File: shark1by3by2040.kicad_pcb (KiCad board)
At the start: 2 copper layers, 35 parts, among them J1 SWD, SW1 SW_USB_BOOT, SW2 SW_Reset, U1 RP2040, U2 W25Q128JVS, U3 NCP1117-3.3_SOT223, Y1 ABLS-12.000MHZ-B4-T

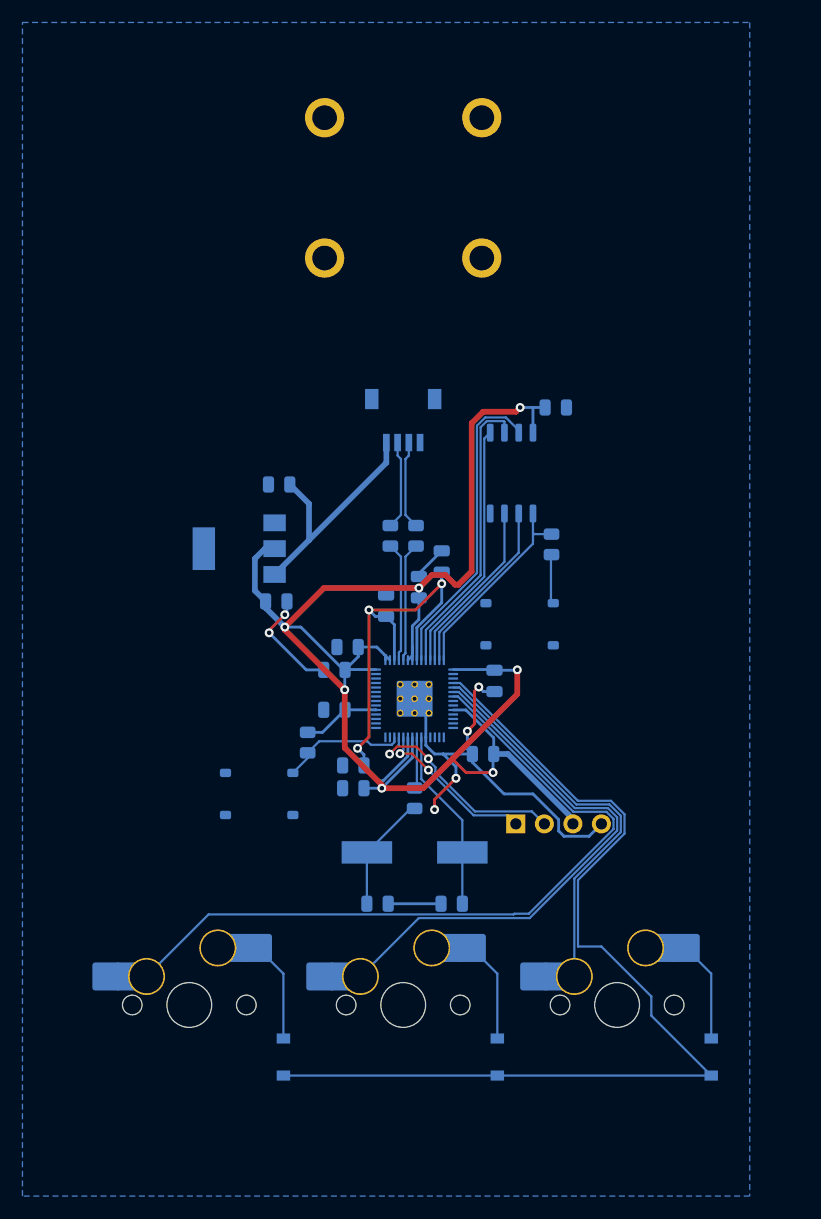
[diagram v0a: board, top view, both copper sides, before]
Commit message: 1by3by2040 rev1
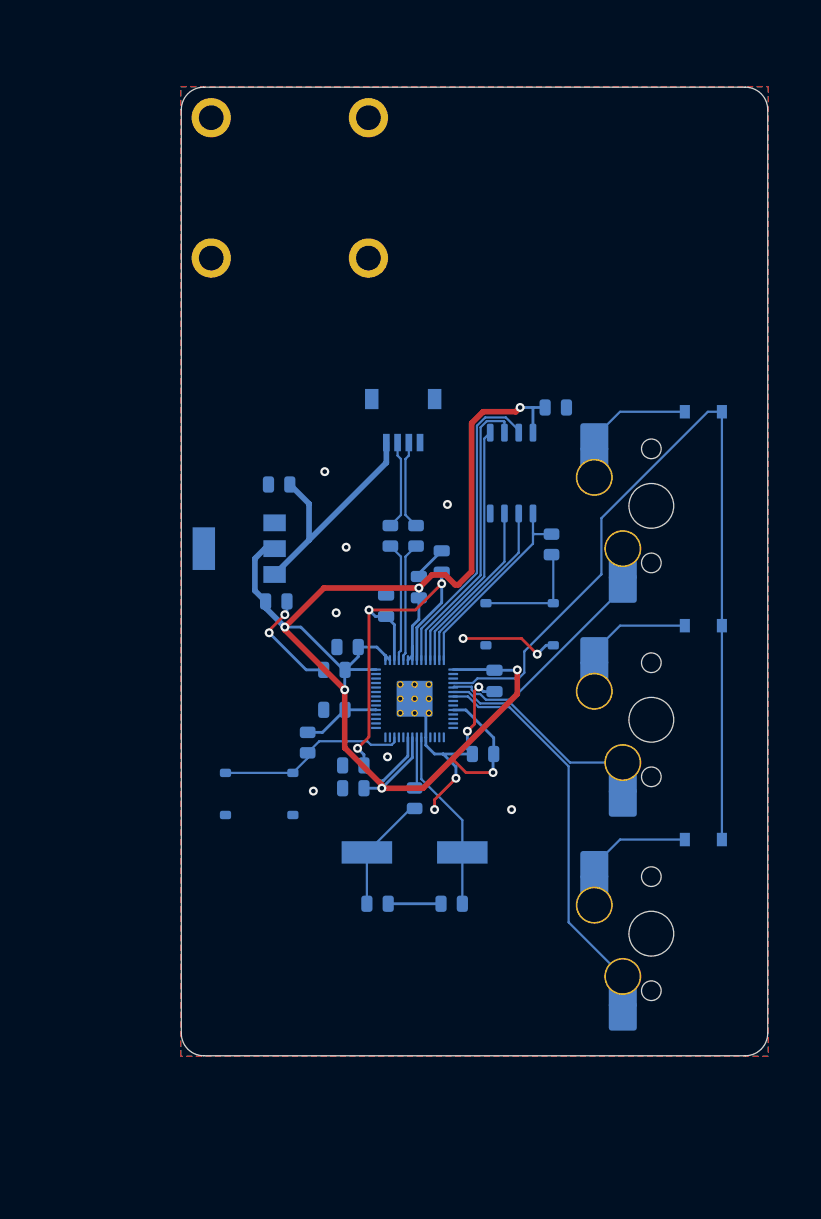
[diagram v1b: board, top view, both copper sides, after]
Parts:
- removed J1: SWD, Connector_PinHeader_2.54mm:PinHeader_1x04_P2.54mm_Vertical
- SW1: value SW_USB_BOOT -> BOOTSEL
- SW2: value SW_Reset -> Reset
- U2: value W25Q128JVS -> W25Q16JVSSIQ
- moved D3 57.5 mm to (200.3, 57.8), turned to 180 degrees
- moved MX3 44.6 mm to (195.7, 66.2), turned to -90 degrees
- moved D2 42.6 mm to (200.3, 76.8), turned to 180 degrees
- moved D1 42.1 mm to (200.3, 95.9), turned to 180 degrees
- moved MX1 41.6 mm to (195.7, 104.3), turned to -90 degrees
- moved MX2 33.7 mm to (195.7, 85.2), turned to -90 degrees
- moved H1 10.1 mm to (163.5, 37.8)
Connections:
- U1 pad 24: Net-(J1-Pad1) -> unconnected-(U1-Pad24)
- U1 pad 25: Net-(J1-Pad2) -> unconnected-(U1-Pad25)
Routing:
- net col0: track 66.7 -> 33.6 mm
- net col1: track 48.7 -> 17.7 mm
- net Net-(J1-Pad2): track 19.1 -> 0.00 mm, vias 2 -> 0
- net col2: track 35.7 -> 19.9 mm
- net Net-(J1-Pad1): track 14.5 -> 0.00 mm, vias 2 -> 0
- net row0: track 89.3 -> 76.1 mm
- net +3V3: track 155.9 -> 145.9 mm
- net GND: track 55.3 -> 48.0 mm, vias 6 -> 15
- net Net-(R3-Pad1): track 4.07 -> 10.2 mm
- net Net-(R5-Pad2): track 11.1 -> 17.1 mm
- added copper zone on F.Cu, net GND
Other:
- board outline added: 52.2 x 86.3 mm

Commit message: 1by3by2040 rev2
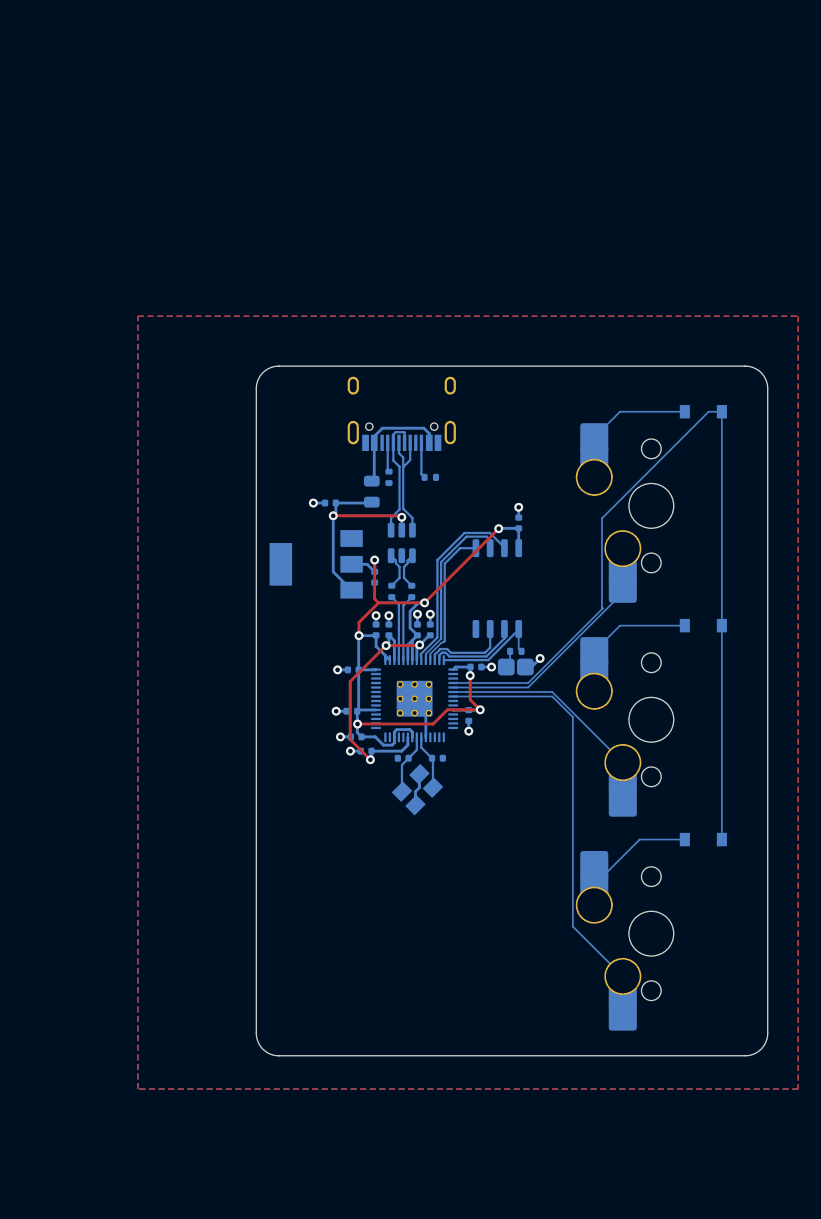
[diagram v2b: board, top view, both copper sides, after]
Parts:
- removed A1: USB, random-keyboard-parts:JST-SR-4
- removed H1: Daughterboard, local:UNIFIED-DAUGHTERBOARD-C3
- removed SW1: BOOTSEL, local:TS-1187A
- removed SW2: Reset, local:TS-1187A
- added F1: 500mA, Fuse:Fuse_0805_2012Metric, B.Cu at (170.8, 64.9)
- added JP1: BOOTSEL, random-keyboard-parts:Jumper-UserFriendly-Small, B.Cu at (183.6, 80.5)
- added U4: USBLC6-2SC6, Package_TO_SOT_SMD:SOT-23-6, B.Cu at (173.5, 69.5)
- added USB1: HRO-TYPE-C-31-M-12, Type-C:HRO-TYPE-C-31-M-12-Assembly, B.Cu at (173.5, 52.9)
- C1, C10, C11, C12, C13, C14, C15, C2, C3, C4, C5, C6, C7: footprint Capacitor_SMD:C_0805_2012Metric -> Capacitor_SMD:C_0402_1005Metric
- C16, C17: value 27pF -> 22pF; footprint Capacitor_SMD:C_0805_2012Metric -> Capacitor_SMD:C_0402_1005Metric
- D1, D2, D3: footprint Diode_SMD:D_SOD-123 -> random-keyboard-parts:D_SOD-123-Pretty
- R1, R2, R3: footprint Resistor_SMD:R_0805_2012Metric -> Resistor_SMD:R_0402_1005Metric
- R4, R5: value 1k -> 5.1k; footprint Resistor_SMD:R_0805_2012Metric -> Resistor_SMD:R_0402_1005Metric
- Y1: value ABLS-12.000MHZ-B4-T -> RH100-12.000-16-3030-TR; footprint Crystal:Crystal_SMD_HC49-SD -> Crystal:Crystal_SMD_3225-4Pin_3.2x2.5mm
- moved R4 28.7 mm to (172.3, 63.6), turned to -90 degrees
- moved R5 26.0 mm to (176.0, 63.6), turned to 0 degrees
- moved C17 13.2 mm to (173.6, 88.6)
- moved C16 13.0 mm to (176.7, 88.6)
- moved C13 10.8 mm to (183.9, 67.7), turned to 90 degrees
- moved U2 10.4 mm to (182.0, 73.5)
- moved R3 10.0 mm to (183.6, 79.1), turned to 0 degrees
- moved C14 9.03 mm to (171.1, 72.5), turned to 90 degrees
- moved U3 7.00 mm to (165.9, 71.4)
- moved C1 6.18 mm to (176.0, 77.2)
- moved Y1 5.59 mm to (174.9, 91.4), turned to 45 degrees
- moved R1 4.97 mm to (174.4, 73.8)
- moved R2 4.95 mm to (172.6, 73.8)
- moved C15 4.86 mm to (167.1, 65.9)
- moved C5 4.58 mm to (169.4, 86.7)
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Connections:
- net /DN renamed Net-(R2-Pad1)
- net /DP renamed Net-(R1-Pad1)
- C16 pad 1: GND -> XIN
- C16 pad 2: Net-(C16-Pad2) -> GND
- C17 pad 1: GND -> XOUT
- C17 pad 2: Net-(C17-Pad2) -> GND
- R4 pad 1: Net-(C17-Pad2) -> Net-(R4-Pad1)
- R4 pad 2: Net-(R4-Pad2) -> GND
- R5 pad 1: +3V3 -> Net-(R5-Pad1)
- R5 pad 2: Net-(R5-Pad2) -> GND
- U1 pad 20: Net-(C16-Pad2) -> XIN
- U1 pad 21: Net-(R4-Pad2) -> XOUT
- U1 pad 26: Net-(R5-Pad2) -> +3V3
- Y1 pad 1: Net-(C17-Pad2) -> XOUT
- Y1 pad 2: Net-(C16-Pad2) -> GND
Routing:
- net +3V3: track 145.9 -> 79.7 mm
- net GND: track 48.0 -> 17.1 mm, vias 15 -> 13
- net +1V1: track 44.8 -> 26.3 mm
- net Net-(R5-Pad2): track 17.1 -> 0.00 mm
- net Net-(C16-Pad2): track 16.3 -> 0.00 mm
- net DN: track 0.00 -> 11.1 mm
- net Net-(U1-Pad51): track 27.4 -> 16.7 mm
- net DP: track 0.00 -> 10.7 mm
- net SCLK: track 26.1 -> 15.5 mm
- net Net-(C17-Pad2): track 10.1 -> 0.00 mm
- net Net-(U1-Pad53): track 22.5 -> 12.6 mm
- net VBUS: track 0.00 -> 9.42 mm
- net Net-(R3-Pad1): track 10.2 -> 1.06 mm
- net SS: track 18.0 -> 9.89 mm
- net Net-(U1-Pad54): track 15.6 -> 7.61 mm
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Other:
- board size 52.2 x 86.3 mm -> 45.5 x 61.4 mm
